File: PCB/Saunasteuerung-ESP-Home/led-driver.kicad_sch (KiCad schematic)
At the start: 13 parts, among them Q4 IRLZ34N, Q7 IRLZ34N, Q8 IRLZ34N, Q9 IRLZ34N, X2 LED's

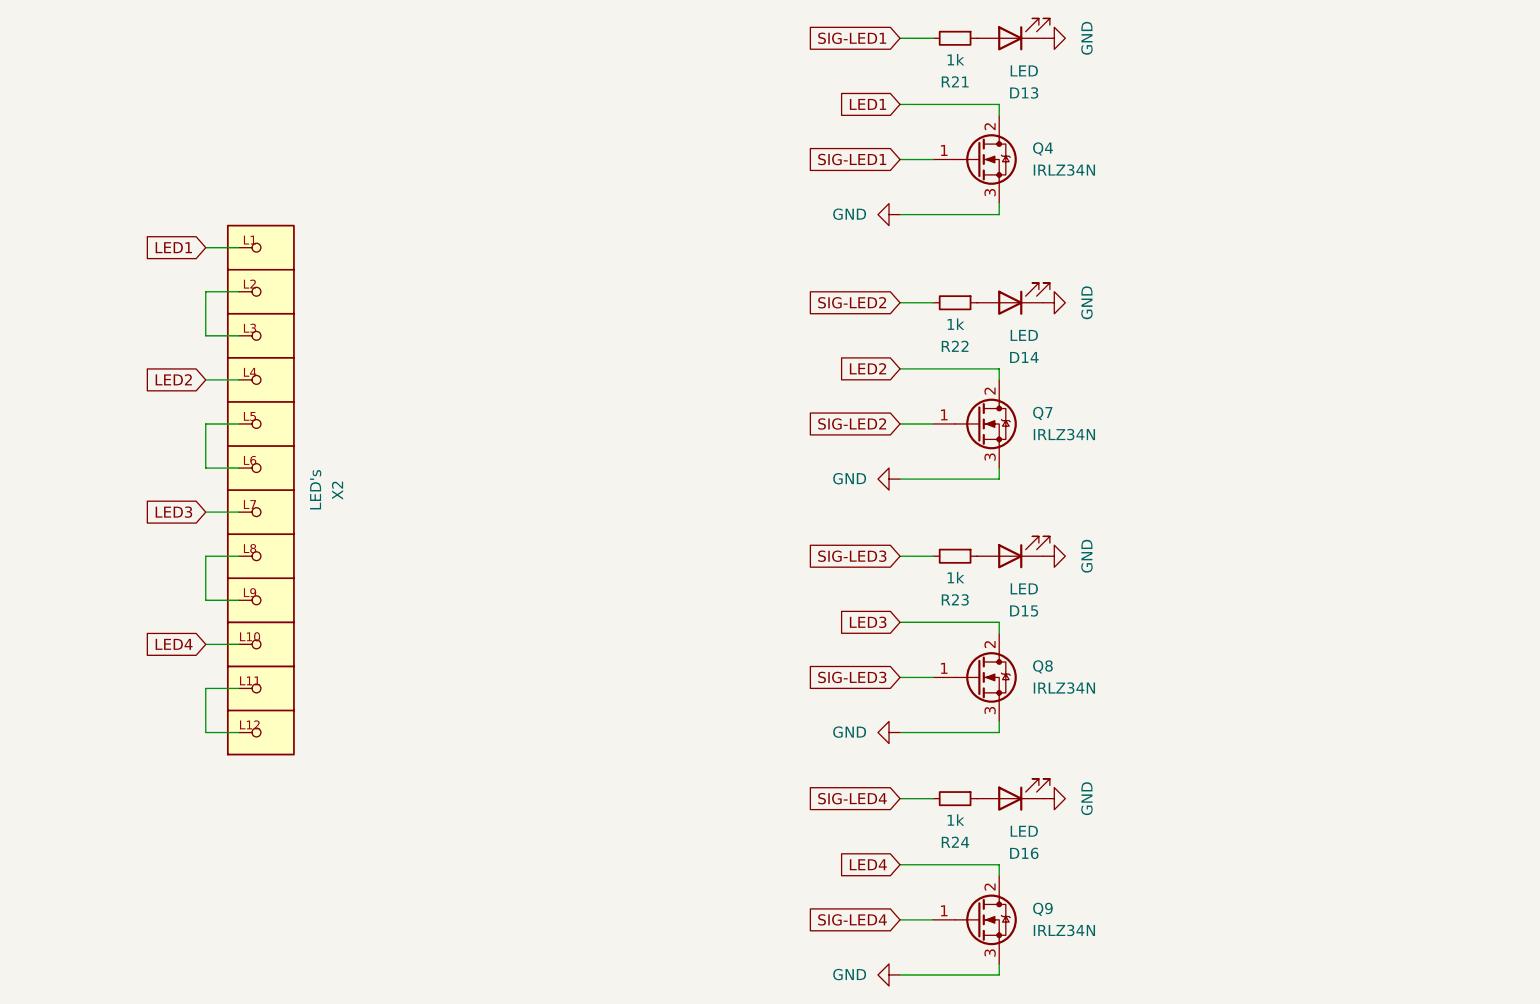
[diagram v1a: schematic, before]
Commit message: V2.0 push
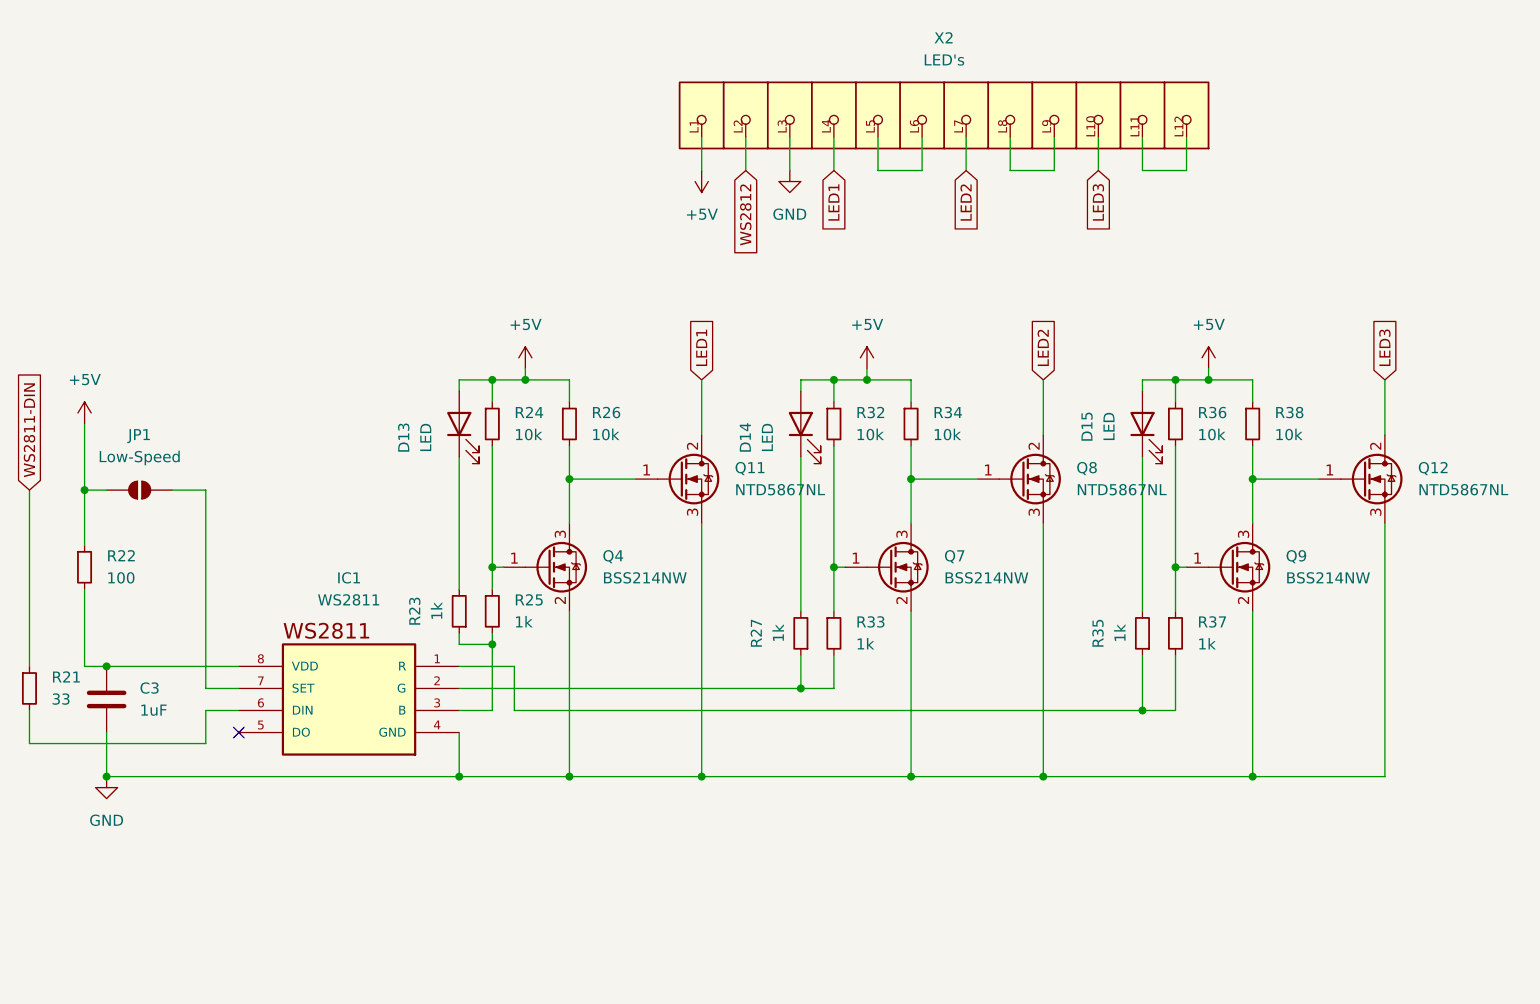
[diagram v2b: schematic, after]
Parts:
- removed D16: LED, LED_SMD:LED_0603_1608Metric, symbol Device:LED
- removed Q4, Q7, Q8, Q9: IRLZ34N, Package_TO_SOT_THT:TO-220-3_Vertical, symbol Transistor_FET:IRLZ34N
- added C3: 1uF, Capacitor_SMD:C_0603_1608Metric, symbol Device:C
- added IC1: WS2811, WS2811:SO08-SKINNYPADS, symbol WS2811:WS2811
- added JP1: Low-Speed, Jumper:SolderJumper-2_P1.3mm_Open_TrianglePad1.0x1.5mm, symbol Jumper:SolderJumper_2_Open
- added Q11, Q12, Q8: NTD5867NL, Package_TO_SOT_SMD:TO-252-2, symbol Transistor_FET:STD7NK40Z
- added Q4, Q7, Q9: BSS214NW, Package_TO_SOT_SMD:SOT-323_SC-70, symbol Transistor_FET:BSS214NW
- added R21: 33, Resistor_SMD:R_0603_1608Metric, symbol Device:R_Small
- added R22: 100, Resistor_SMD:R_0603_1608Metric, symbol Device:R_Small
- added R25, R33, R37: 1k, Resistor_SMD:R_0603_1608Metric, symbol Device:R_Small
- added R26, R32, R34, R36, R38: 10k, Resistor_SMD:R_0603_1608Metric, symbol Device:R_Small
- R24: value 1k -> 10k
- renumbered R21 to R23, R22 to R27, R23 to R35
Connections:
- net LED4 is gone; now on net LED3: X2.L10
- net GND: now also X2.L3, C3.2, IC1.4 (GND), Q11.3 (S), Q12.3 (S), Q4.2 (S), Q7.2 (S), Q8.3 (S), Q9.2 (S); no longer D13.1 (K), D14.1 (K), D15.1 (K)
- net LED1: now also X2.L4, Q11.2 (D); no longer X2.L1
- net LED2: now also X2.L7, Q8.2 (D); no longer X2.L4
- net LED3: now also Q12.2 (D); no longer X2.L7
- net at R23.1: now also IC1.3 (B), R25.2; no longer D13.2 (A)
- net +5V: now reaches R24.1
- net +5V: now also D13.2 (A), D14.2 (A), D15.2 (A), X2.L1, JP1.2 (B), R22.1, R26.1, R32.1, R34.1, R36.1, R38.1
- net at R35.1: now also IC1.1 (R), R37.2; no longer D15.2 (A)
- net at R27.1: now also IC1.2 (G), R33.2; no longer D14.2 (A)
- net WS2812: now reaches X2.L2
- net WS2812: no longer X2.L3
- net SIG-LED1: no longer names the net of R23.2
- net SIG-LED1: now also D13.1 (K)
- net SIG-LED2: no longer names the net of R27.2
- net SIG-LED2: now also D14.1 (K)
- net SIG-LED3: no longer names the net of R35.2
- net SIG-LED3: now also D15.1 (K)
- net SIG-LED4: no longer names the net of R24.2
- net SIG-LED4: now also Q4.1 (G), R25.1
- new net: IC1.6 (DIN), R21.2
- new net: Q9.1 (G), R36.2, R37.1
- new net: IC1.7 (SET), JP1.1 (A)
- new net: Q12.1 (G), Q9.3 (D), R38.2
- new net: Q11.1 (G), Q4.3 (D), R26.2
- new net: C3.1, IC1.8 (VDD), R22.2
- new net: Q7.3 (D), Q8.1 (G), R34.2
- new net: Q7.1 (G), R32.2, R33.1
- new net WS2811-DIN: R21.1
- no-connect marks 0 -> 1
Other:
- moved on the sheet: D13, D14, D15, R23, R27, R35, X2
